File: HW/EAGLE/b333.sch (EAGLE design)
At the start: 187 parts, among them Q5 NMOSD, X1 USB MICRO

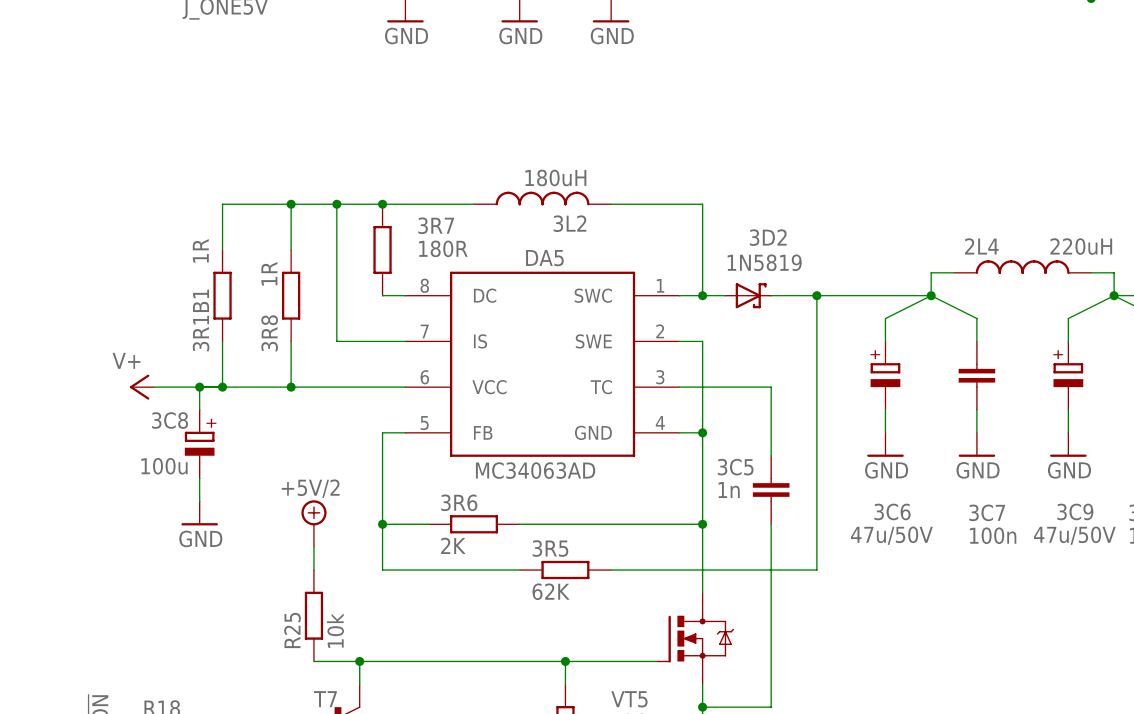
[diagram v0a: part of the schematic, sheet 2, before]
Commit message: .
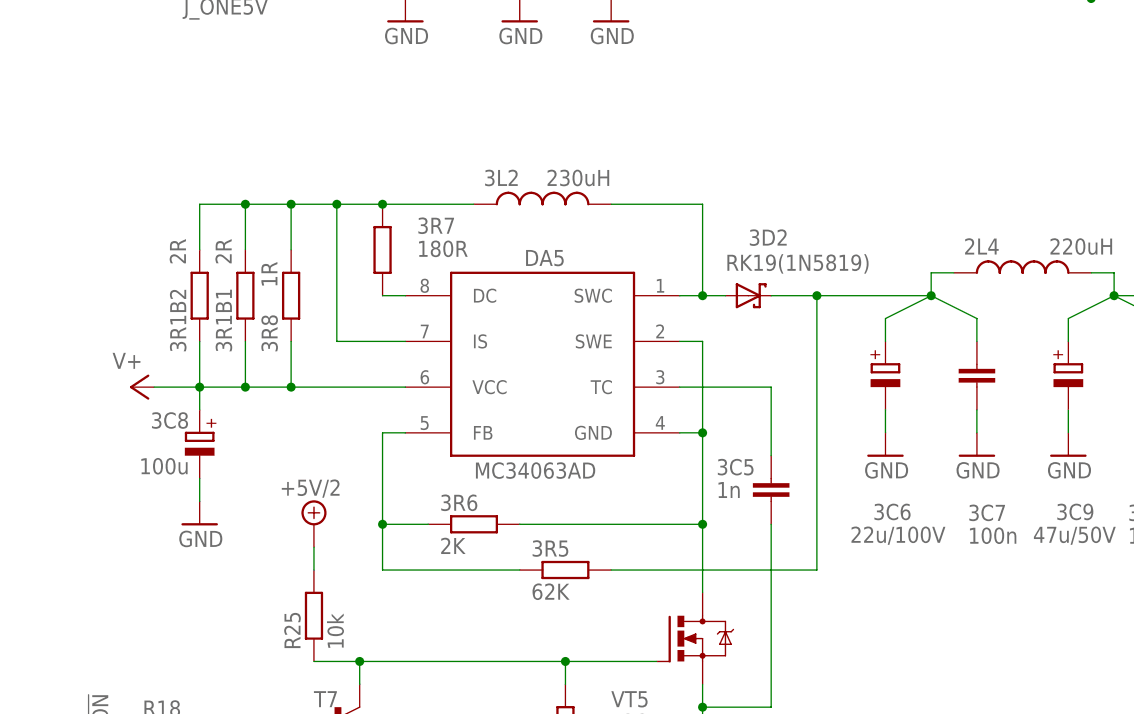
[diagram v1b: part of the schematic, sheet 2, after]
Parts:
- added 3R1B2: 2R, resistor:R-EU_R0805
- 1C13: device resistor:C-EUC0805 -> resistor:C-EUC0805K
- 3C6: value 47u/50V -> 22u/100V
- 3D2: value 1N5819 -> RK19(1N5819)
- 3L2: value 180uH -> 230uH
- 3R1B1: value 1R -> 2R
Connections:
- net N$54: now also 3R1B2.2
- net V+: now also 3R1B2.1
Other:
- moved on the sheet: 3R1B1
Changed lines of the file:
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@@
 <part name="ZEN_A1" library="pinhead" deviceset="PINHD-1X1" device=""/>
 <part name="DA5" library="mc34063-2" deviceset="MC34063" device="AD"/>
-<part name="3L2" library="rcl" deviceset="L-US" device="6000-XXX-RC" value="180uH"/>
-<part name="3D2" library="diode" deviceset="SCHOTTKY-DIODE" device="SMD" value="1N5819"/>
+<part name="3L2" library="rcl" deviceset="L-US" device="6000-XXX-RC" value="230uH"/>
+<part name="3D2" library="diode" deviceset="SCHOTTKY-DIODE" device="SMD" value="RK19(1N5819)"/>
 <part name="3C5" library="resistor" deviceset="C-EU" device="C0805K" value="1n"/>
-<part name="3C6" library="resistor" deviceset="CPOL-EU" device="E2.5-6" value="47u/50V"/>
+<part name="3C6" library="resistor" deviceset="CPOL-EU" device="E2.5-6" value="22u/100V"/>
 <part name="3C7" library="resistor" deviceset="C-EU" device="C0805K" value="100n"/>
 <part name="U$31" library="lib-user" deviceset="GND" device=""/>
@@
 <part name="U$34" library="lib-user" deviceset="GND" device=""/>
 <part name="R8" library="resistor" deviceset="R-EU_" device="R0805" value="100k"/>
-<part name="3R1B1" library="resistor" deviceset="R-EU_" device="R0805" value="1R"/>
+<part name="3R1B1" library="resistor" deviceset="R-EU_" device="R0805" value="2R"/>
 <part name="SUPPLY6" library="supply2" deviceset="V+" device=""/>
 <part name="2L4" library="rcl" deviceset="L-US" device="6000-XXX-RC" value="220uH"/>
@@
 <part name="1R25" library="resistor" deviceset="R-EU_" device="R0805" value="2K2"/>
 <part name="1L2" library="rcl" deviceset="L-US" device="IRF-24" value="10mkhn"/>
-<part name="1C13" library="resistor" deviceset="C-EU" device="C0805" value="100n"/>
+<part name="1C13" library="resistor" deviceset="C-EU" device="C0805K" value="100n"/>
 <part name="U$54" library="lib-user" deviceset="GND" device=""/>
 <part name="4Y3" library="relay_ussr" deviceset="РЭС55" device="А" value="РЭС55А"/>
@@
 <part name="T7" library="transistor" deviceset="*-NPN-" device="TO92-ECB"/>
 <part name="U$12" library="lib-user" deviceset="GND" device=""/>
+<part name="3R1B2" library="resistor" deviceset="R-EU_" device="R0805" value="2R"/>
 </parts>
 <sheets>
@@
 <attribute name="VALUE" x="119.38" y="53.34" size="1.778" layer="96"/>
 </instance>
-<instance part="3L2" gate="G$1" x="127" y="83.82" rot="R90"/>
+<instance part="3L2" gate="G$1" x="127" y="83.82" smashed="yes" rot="R90">
+<attribute name="NAME" x="124.46" y="87.63" size="1.778" layer="95" rot="R180"/>
+<attribute name="VALUE" x="134.62" y="87.63" size="1.778" layer="96" rot="R180"/>
+</instance>
 <instance part="3D2" gate="G$1" x="149.86" y="73.66" smashed="yes">
 <attribute name="NAME" x="149.86" y="79.2226" size="1.778" layer="95"/>
@@
 <instance part="U$34" gate="G$1" x="144.78" y="25.4"/>
 <instance part="R8" gate="G$1" x="129.54" y="25.4" rot="R90"/>
-<instance part="3R1B1" gate="G$1" x="91.44" y="73.66" smashed="yes" rot="R90">
-<attribute name="NAME" x="89.9414" y="67.31" size="1.778" layer="95" rot="R90"/>
-<attribute name="VALUE" x="88.138" y="80.01" size="1.778" layer="96" rot="R270"/>
+<instance part="3R1B1" gate="G$1" x="93.98" y="73.66" smashed="yes" rot="R90">
+<attribute name="NAME" x="92.4814" y="67.31" size="1.778" layer="95" rot="R90"/>
+<attribute name="VALUE" x="90.678" y="80.01" size="1.778" layer="96" rot="R270"/>
 </instance>
 <instance part="SUPPLY6" gate="1" x="81.28" y="63.5" smashed="yes" rot="R90">
@@
 </instance>
 <instance part="U$12" gate="G$1" x="106.68" y="15.24"/>
+<instance part="3R1B2" gate="G$1" x="88.9" y="73.66" smashed="yes" rot="R90">
+<attribute name="NAME" x="87.4014" y="67.31" size="1.778" layer="95" rot="R90"/>
+<attribute name="VALUE" x="85.598" y="80.01" size="1.778" layer="96" rot="R270"/>
+</instance>
 </instances>
 <busses>
@@
 <wire x1="111.76" y1="63.5" x2="99.06" y2="63.5" width="0.1524" layer="91"/>
 <pinref part="SUPPLY6" gate="1" pin="V+"/>
-<wire x1="99.06" y1="63.5" x2="88.9" y2="63.5" width="0.1524" layer="91"/>
+<wire x1="99.06" y1="63.5" x2="93.98" y2="63.5" width="0.1524" layer="91"/>
 <wire x1="99.06" y1="68.58" x2="99.06" y2="63.5" width="0.1524" layer="91"/>
 <junction x="99.06" y="63.5"/>
-<wire x1="91.44" y1="68.58" x2="91.44" y2="63.5" width="0.1524" layer="91"/>
-<wire x1="91.44" y1="63.5" x2="88.9" y2="63.5" width="0.1524" layer="91"/>
+<wire x1="93.98" y1="68.58" x2="93.98" y2="63.5" width="0.1524" layer="91"/>
+<wire x1="93.98" y1="63.5" x2="88.9" y2="63.5" width="0.1524" layer="91"/>
 <wire x1="88.9" y1="63.5" x2="83.82" y2="63.5" width="0.1524" layer="91"/>
-<junction x="91.44" y="63.5"/>
+<junction x="93.98" y="63.5"/>
+<pinref part="3R1B2" gate="G$1" pin="1"/>
+<wire x1="88.9" y1="68.58" x2="88.9" y2="63.5" width="0.1524" layer="91"/>
 </segment>
 </net>
@@
 <wire x1="104.14" y1="83.82" x2="99.06" y2="83.82" width="0.1524" layer="91"/>
 <wire x1="99.06" y1="83.82" x2="99.06" y2="78.74" width="0.1524" layer="91"/>
-<wire x1="91.44" y1="78.74" x2="91.44" y2="83.82" width="0.1524" layer="91"/>
-<wire x1="91.44" y1="83.82" x2="99.06" y2="83.82" width="0.1524" layer="91"/>
+<wire x1="93.98" y1="78.74" x2="93.98" y2="83.82" width="0.1524" layer="91"/>
+<wire x1="93.98" y1="83.82" x2="99.06" y2="83.82" width="0.1524" layer="91"/>
 <junction x="99.06" y="83.82"/>
 <junction x="109.22" y="83.82"/>
-</segment>
-</net>
+<pinref part="3R1B2" gate="G$1" pin="2"/>
+<wire x1="88.9" y1="78.74" x2="88.9" y2="83.82" width="0.1524" layer="91"/>
+<wire x1="88.9" y1="83.82" x2="93.98" y2="83.82" width="0.1524" layer="91"/>
+<junction x="93.98" y="83.82"/>
+</segment>
+</net>
